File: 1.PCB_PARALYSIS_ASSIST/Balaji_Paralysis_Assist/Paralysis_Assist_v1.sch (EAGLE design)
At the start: 20 parts, among them IC2 7805TV, U1 ZC563900

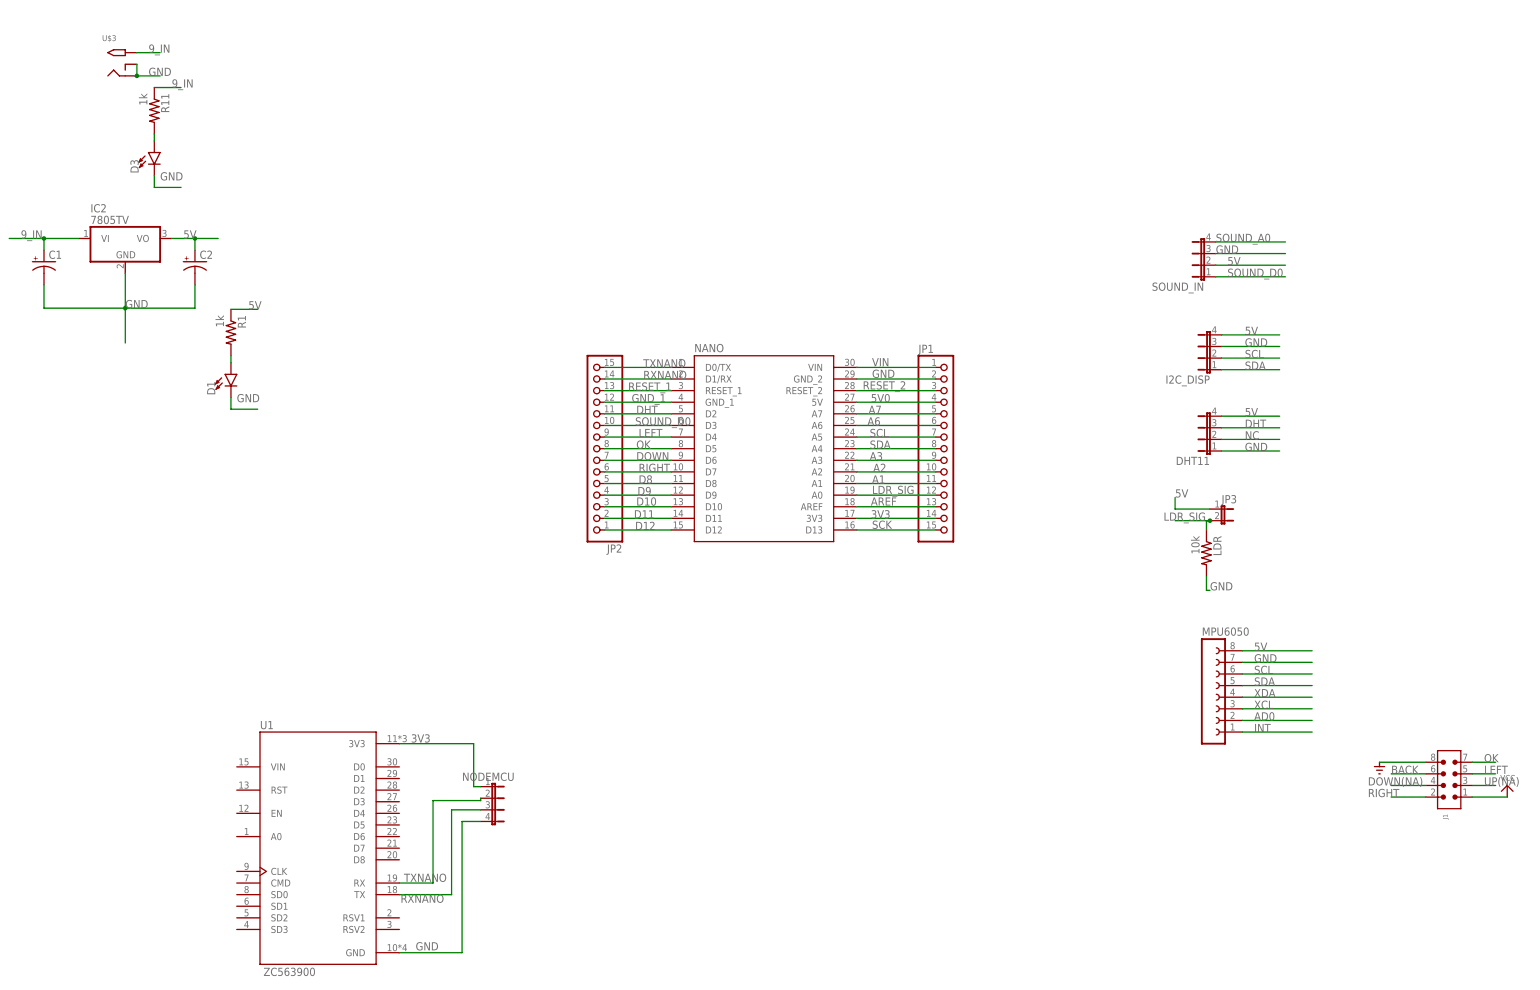
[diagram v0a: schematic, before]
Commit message: initial_commit
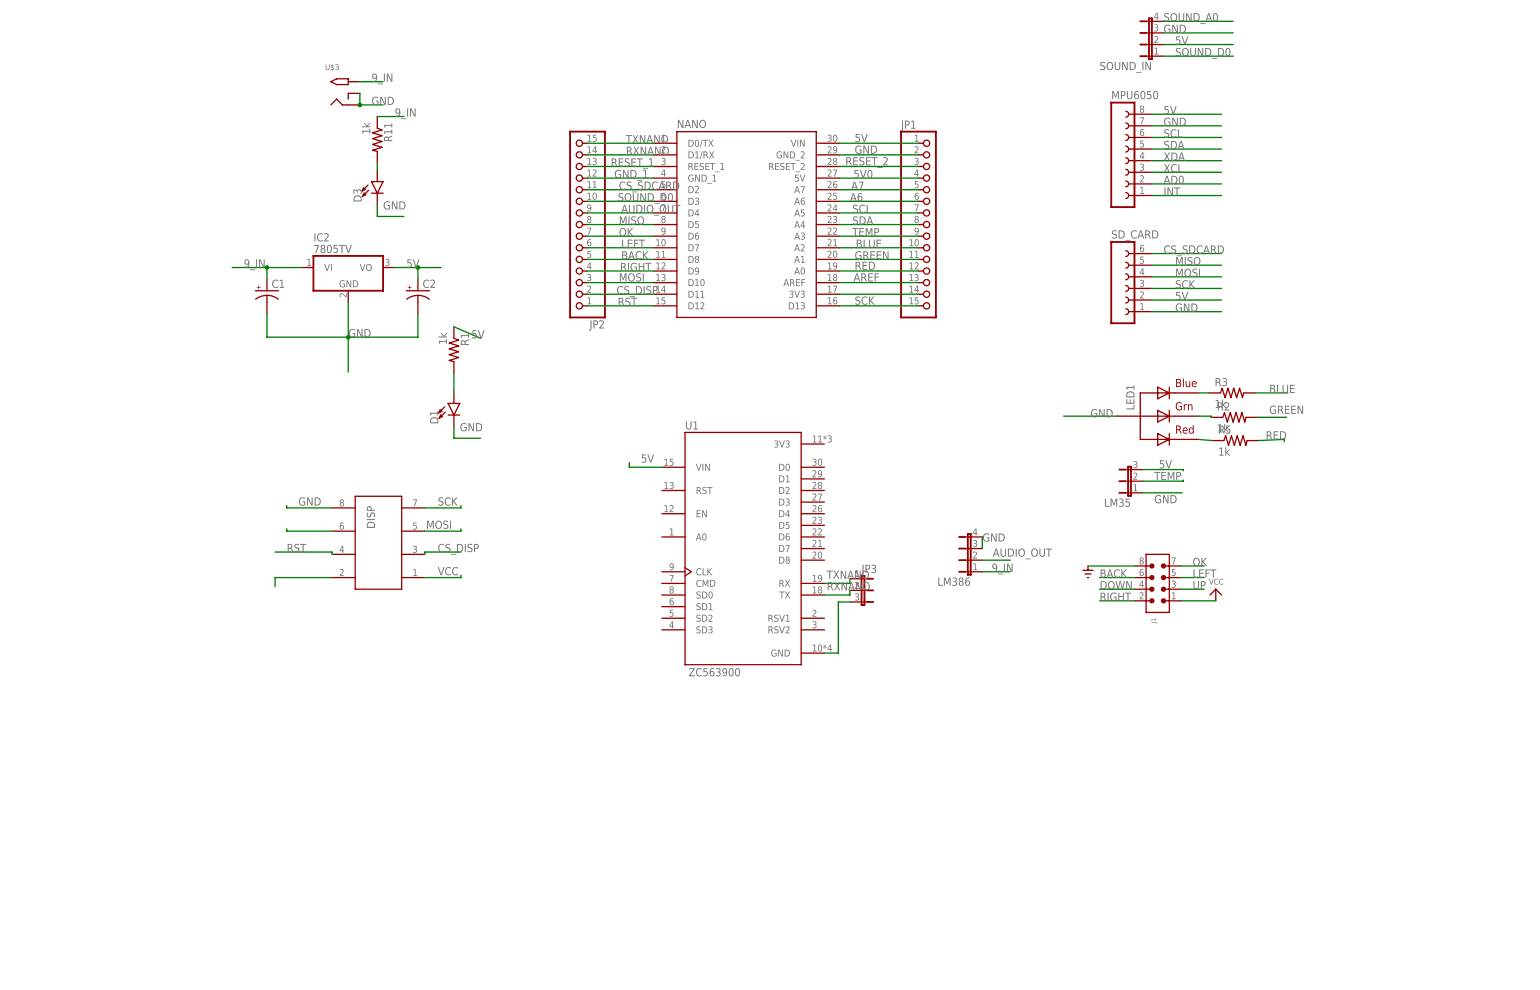
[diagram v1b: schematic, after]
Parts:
- removed DHT11, I2C_DISP, NODEMCU: (no value), jumper:JP4E
- removed LDR: 10k, adafruit:R-US_M0805
- added DISP: (no value), Wurth_Elektronik_Electromechanic_Wire_to_Board_Connectors_rev19a:612008235121
- added LED1: RGBLED_CA-5MM, adafruit:RGBLED_CA-5MM
- added LM35: (no value), jumper:JP2E
- added LM386: (no value), jumper:JP4E
- added R2, R3, R5: 1k, adafruit:R-US_M0805
- added SD_CARD: (no value), con-lsta:FE06-1
- JP3: device jumper:JP1E -> jumper:JP2W
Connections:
- net UP(NA) renamed UP
- removed net 3V3: JP1.14, NANO.3V3, NODEMCU.1, U1.3V3
- removed net A1: JP1.11, NANO.A1
- removed net A2: JP1.10, NANO.A2
- removed net A3: JP1.9, NANO.A3
- removed net D10: JP2.3, NANO.D10
- removed net D11: JP2.2, NANO.D11
- removed net D12: JP2.1, NANO.D12
- removed net D8: JP2.5, NANO.D8
- removed net D9: JP2.4, NANO.D9
- removed net DHT: DHT11.3, JP2.11, NANO.D2
- removed net DOWN(NA): J1.4
- removed net LDR_SIG: JP1.12, JP3.2, LDR.1, NANO.A0
- removed net NC: DHT11.2
- removed net VIN: JP1.1, NANO.VIN
- new net AUDIO_OUT: JP2.9, LM386.2, NANO.D4
- new net BLUE: JP1.10, NANO.A2, R3.2
- new net CS_DISP: DISP.3, JP2.2, NANO.D11
- new net CS_SDCARD: JP2.11, NANO.D2, SD_CARD.6
- new net GREEN: JP1.11, NANO.A1, R2.2
- new net MISO: JP2.8, NANO.D5, SD_CARD.5
- new net MOSI: DISP.5, JP2.3, NANO.D10, SD_CARD.4
- new net N$1: DISP.2
- new net N$10: JP3.3, U1.GND
- new net N$4: LED1.BLUE, R3.1
- new net N$5: DISP.6
- new net N$6: LED1.GREEN, R2.1
- new net N$7: LED1.RED, R5.1
- new net N$8: JP1.14, NANO.3V3
- new net RED: JP1.12, NANO.A0, R5.2
- new net RST: DISP.4, JP2.1, NANO.D12
- new net TEMP: JP1.9, LM35.2, NANO.A3
- net 5V: now also JP1.1, LM35.3, NANO.VIN, SD_CARD.2, U1.VIN; no longer DHT11.4, I2C_DISP.4, JP3.1
- net 9_IN: now also LM386.1
- net BACK: now also JP2.5, NANO.D8
- net DOWN: now also J1.4; no longer JP2.7, NANO.D6
- net GND: now also DISP.8, LED1.VCC, LM35.1, LM386.3, LM386.4, SD_CARD.1; no longer DHT11.1, I2C_DISP.3, LDR.2, NODEMCU.4, U1.GND
- net LEFT: now also JP2.6, NANO.D7; no longer JP2.9, NANO.D4
- net OK: now also JP2.7, NANO.D6; no longer JP2.8, NANO.D5
- net RIGHT: now also JP2.4, NANO.D9; no longer JP2.6, NANO.D7
- net RXNANO: now also JP3.2; no longer NODEMCU.3
- net SCK: now also DISP.7, SD_CARD.3
- net SCL: no longer I2C_DISP.2
- net SDA: no longer I2C_DISP.1
- net TXNANO: now also JP3.1; no longer NODEMCU.2
- net VCC: now also DISP.1
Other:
- moved on the sheet: C1, C2, D1, D3, IC2, J1, JP1, JP2, MPU6050, NANO, R1, R11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
